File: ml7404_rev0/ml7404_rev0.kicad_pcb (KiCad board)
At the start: 4 copper layers, 53.7 x 30.5 mm, 97 parts, among them CN1 MHF-SW23, 20549-001E, CN2 MHF1, 20279-001E-03, U1 SKY13438-374LF, U2 ML7404, U3 BRCB032GWZ-3, U4 BH18PB1WFV

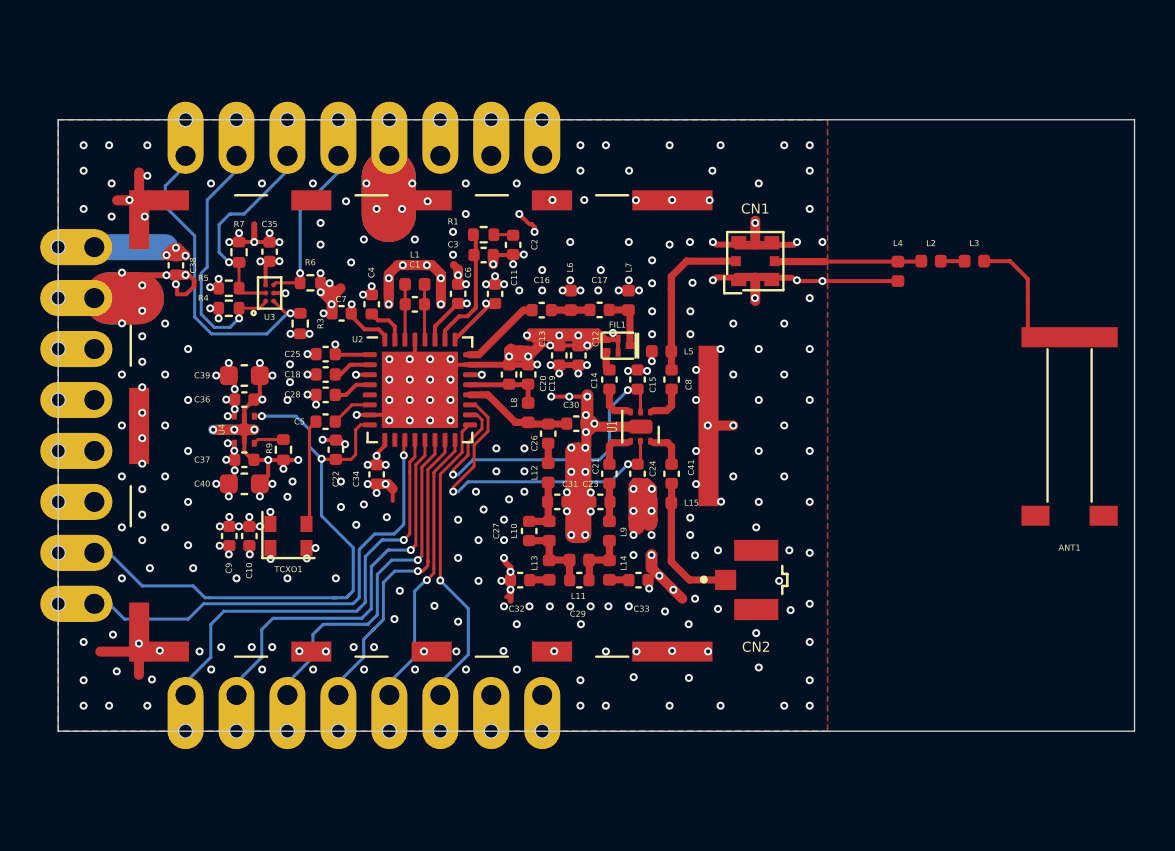
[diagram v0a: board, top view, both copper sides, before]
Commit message: pre layout2
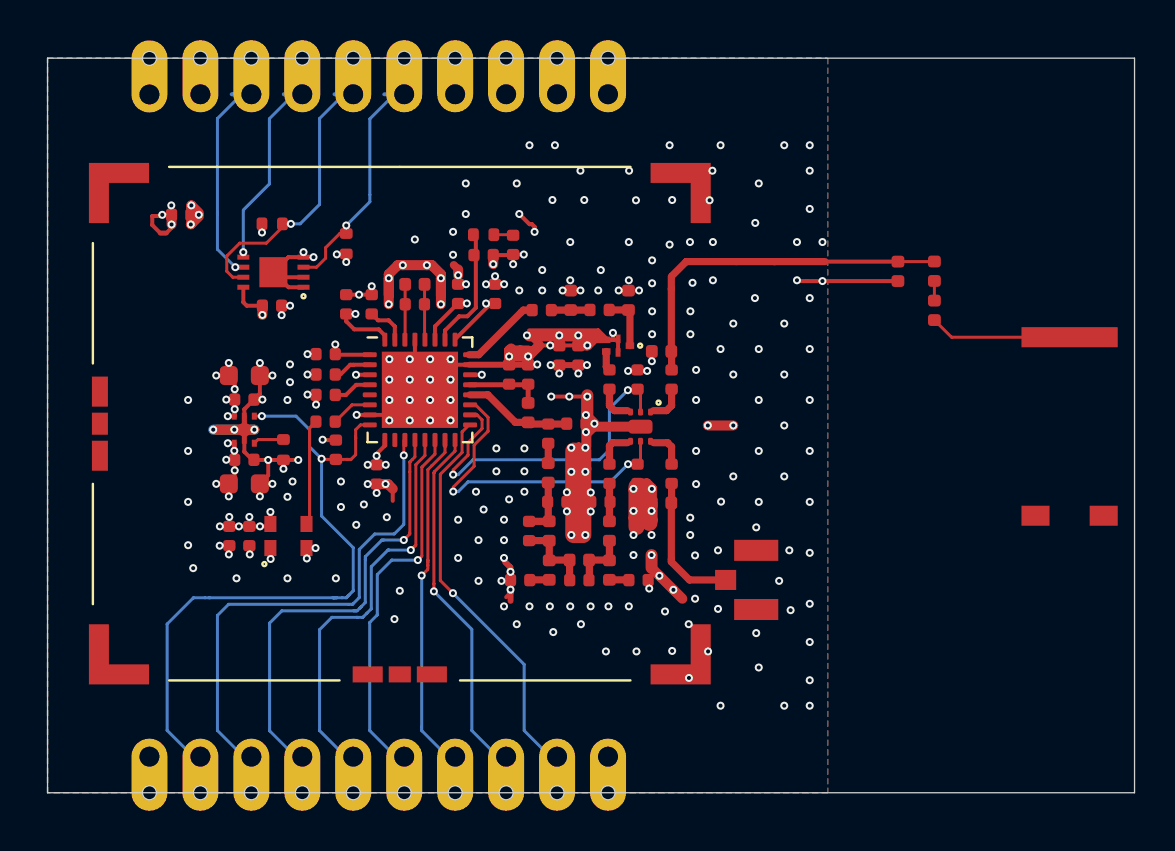
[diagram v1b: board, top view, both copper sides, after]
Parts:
- removed CN1: MHF-SW23, 20549-001E, ml7404_module:IPEX_20549-001E
- removed PIN21, PIN22, PIN23, PIN24: Conn_01x01, ml7404_module:terminal
- removed R3, R4, R7: 10kΩ, Resistor_SMD:R_0402_1005Metric
- removed RF_Shield1: RF_Sheild_pre, ml7404_module:RF_Shield_pre_29.85x24.0mm
- added CL1: UTC(RF_Shield_Clip), ml7404_module:UTC_RF_Shield_Clip, F.Cu at (117.7, 97.7)
- added CL2: UTC(RF_Shield_Clip), ml7404_module:UTC_RF_Shield_Clip, F.Cu at (132.6, 110.2)
- added RF_shield1: 1500_RF_shield_soldered_recess, ml7404_module:1500_RF_Shield_soldered_30mmx25mm, F.Cu at (132.6, 97.7)
- C1, C10, C11, C12, C13, C14, C15, C16, C17, C18, C19, C2, C20, C21, C22, C23, C24, C25, C26, C27, C28, C29, C3, C30, C31, C32, C33, C34, C35, C36, C37, C38, C4, C41, C5, C6, C7, C8, C9: footprint Capacitor_SMD:C_0402_1005Metric -> ml7404_module:C_0402_1005Metric
- C39, C40: footprint Capacitor_SMD:C_0603_1608Metric -> ml7404_module:C_0603_1608Metric
- L1, L10, L11, L12, L13, L14, L15, L2, L3, L4, L5, L6, L7, L8, L9: footprint Inductor_SMD:L_0402_1005Metric -> ml7404_module:L_0402_1005Metric
- R1, R6, R9: footprint Resistor_SMD:R_0402_1005Metric -> ml7404_module:R_0402_1005Metric
- R5: value N.M. -> 10kΩ; footprint Resistor_SMD:R_0402_1005Metric -> ml7404_module:R_0402_1005Metric
- U3: value BRCB032GWZ-3 -> BR24GxxNUXxx; footprint ml7404_module:BRCB032GWZ-3 -> ml7404_module:BR24GxxNUXxx
- moved PIN11 20.5 mm to (120.1, 114.3), turned to 270 degrees
- moved PIN12 18.5 mm to (122.7, 114.3), turned to 270 degrees
- moved PIN16 17.2 mm to (132.8, 114.3), turned to 270 degrees
- moved PIN13 17.1 mm to (125.2, 114.3), turned to 270 degrees
- moved PIN15 16.4 mm to (130.3, 114.3), turned to 270 degrees
- moved PIN14 16.4 mm to (127.7, 114.3), turned to 270 degrees
- moved PIN17 13.8 mm to (135.4, 114.3)
- moved PIN18 13.8 mm to (137.9, 114.3)
- moved PIN19 13.8 mm to (140.4, 114.3)
- moved PIN20 13.8 mm to (143.0, 114.3)
- moved PIN10 10.5 mm to (120.1, 81.3), turned to 90 degrees
- moved PIN9 9.28 mm to (122.7, 81.3), turned to 90 degrees
- moved PIN1 4.49 mm to (143.0, 81.3)
- moved PIN2 4.49 mm to (140.4, 81.3)
- moved PIN3 4.49 mm to (137.9, 81.3)
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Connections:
- L2 pad 1: Net-(CN1-PadB) -> Net-(C8-Pad1)
- L4 pad 1: Net-(CN1-PadB) -> Net-(C8-Pad1)
- PIN1 pad 1: Net-(PIN1-Pad1) -> GND
- PIN11 pad 1: Net-(PIN11-Pad1) -> GND
- PIN12 pad 1: Net-(PIN12-Pad1) -> RESETN
- PIN13 pad 1: Net-(PIN13-Pad1) -> REGPDIN
- PIN14 pad 1: Net-(PIN14-Pad1) -> SDO
- PIN15 pad 1: RESETN -> SCLK
- PIN16 pad 1: REGPDIN -> SCEN
- PIN17 pad 1: SDO -> SDI
- PIN18 pad 1: SCLK -> GPIO0
- PIN19 pad 1: SCEN -> GPIO1
- PIN20 pad 1: SDI -> GND
- PIN7 pad 1: SCL -> SDA
- PIN8 pad 1: SDA -> SCL
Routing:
- net GND: track 166.0 -> 128.8 mm, vias 348 -> 259
- net +3V3: track 132.7 -> 101.1 mm, vias 26 -> 20
- net Net-(C8-Pad1): track 8.20 -> 18.1 mm
- net Net-(CN1-PadB): track 7.34 -> 0.00 mm
- net SDA: track 16.2 -> 9.21 mm
- net GPIO1: track 16.0 -> 19.5 mm
- net GPIO0: track 14.2 -> 17.5 mm
- net WP: track 10.3 -> 13.6 mm
- net SCL: track 13.0 -> 10.2 mm
- net A2: track 8.48 -> 11.2 mm
- net Net-(ANT1-Pad1): track 7.54 -> 9.17 mm
- net RESETN: track 32.4 -> 33.8 mm
- net SDI: track 16.7 -> 17.3 mm
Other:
- board size 53.7 x 30.5 mm -> 54.2 x 36.6 mm
- rule pad_to_mask_clearance: 0.05 -> 0
